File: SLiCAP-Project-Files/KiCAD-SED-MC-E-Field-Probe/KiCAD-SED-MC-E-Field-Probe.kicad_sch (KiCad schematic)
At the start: 1 part

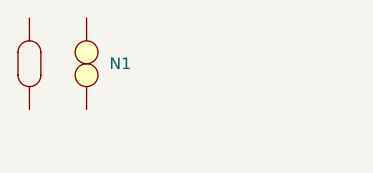
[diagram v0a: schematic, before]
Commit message: FirstAGAIN
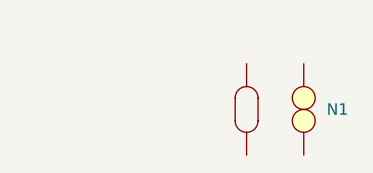
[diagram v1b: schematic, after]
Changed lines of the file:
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@@
 	(symbol
 		(lib_id "SLiCAP:N")
-		(at 95.25 72.39 0)
+		(at 119.38 77.47 0)
 		(unit 1)
 		(exclude_from_sim no)
@@
 		(fields_autoplaced yes)
 		(property "Reference" "N1"
-			(at 97.79 72.3898 0)
+			(at 121.92 77.4698 0)
 			(effects
 				(font
@@
 		)
 		(property "Value" "~"
-			(at 101.6 73.025 0)
+			(at 125.73 78.105 0)
 			(effects
 				(font
@@
 		)
 		(property "Footprint" ""
-			(at 95.25 73.66 0)
+			(at 119.38 78.74 0)
 			(effects
 				(font
@@
 		)
 		(property "Datasheet" ""
-			(at 95.25 73.66 0)
+			(at 119.38 78.74 0)
 			(effects
 				(font
@@
 		)
 		(property "Description" "Nullor"
-			(at 100.33 76.454 0)
+			(at 124.46 81.534 0)
 			(effects
 				(font
@@
 		)
 		(property "model" "N"
-			(at 97.155 74.295 0)
+			(at 121.285 79.375 0)
 			(show_name yes)
 			(effects
@@
 			)
 		)
+		(pin "4"
+		)
+		(pin "3"
+		)
 		(pin "1"
 		)
 		(pin "2"
 		)
-		(pin "4"
-		)
-		(pin "3"
-		)
 		(instances
